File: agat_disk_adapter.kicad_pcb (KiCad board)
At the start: 2 copper layers, 53.3 x 61 mm, 18 parts, among them J1 IDC‐20, J2 IDC‐20, J3 IDC‐34, J4 IDC‐10, J5 KK‐4

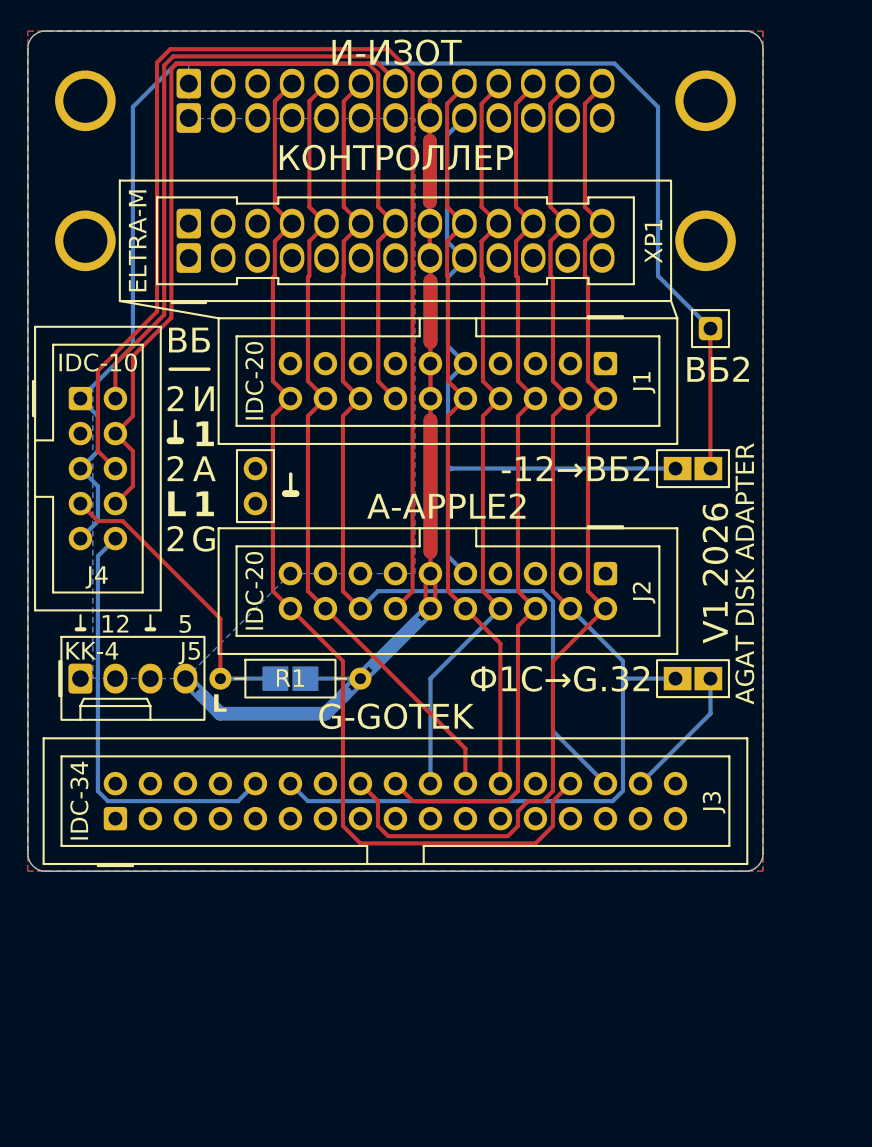
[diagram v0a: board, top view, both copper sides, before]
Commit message: refactor: move PCB to sheet center
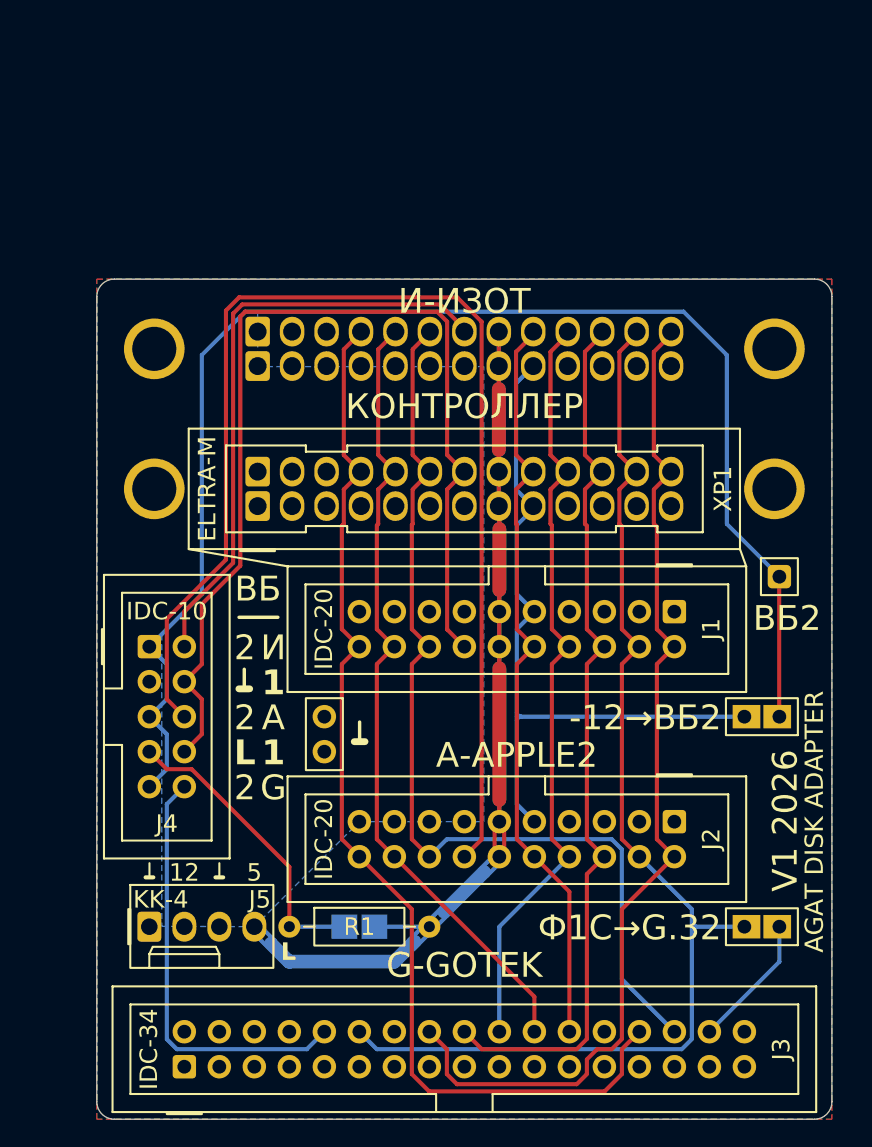
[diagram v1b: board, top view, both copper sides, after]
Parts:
- moved G*** 18.7 mm to (51.9, 58.9)
- moved G*** 18.7 mm to (51.7, 66.0)
- moved G*** 18.7 mm to (95.2, 58.9)
- moved G*** 18.7 mm to (52.3, 97.9)
- moved J1 18.7 mm to (88.8, 81.5)
- moved J2 18.7 mm to (88.8, 96.7)
- moved J3 18.7 mm to (53.3, 114.5)
- moved J4 18.7 mm to (50.7, 84.0)
- moved J5 18.7 mm to (50.7, 104.4)
- moved JP1 18.7 mm to (96.4, 89.1)
- moved JP2 18.7 mm to (96.4, 104.4)
- moved JP3 18.7 mm to (63.4, 89.1)
- moved R1 18.7 mm to (60.9, 104.4)
- moved XP1 18.7 mm to (73.6, 71.3)
- moved XS1 18.7 mm to (73.6, 61.2)
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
